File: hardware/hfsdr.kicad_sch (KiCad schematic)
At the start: 8 parts, among them J1 USB_C_Receptacle_USB2.0_16P, U1 SN74CBT3253, U2 XLV320ADC6120IRTER, U3 CH32V30xFxPx, U4 XC6206PxxxMR, Y1 Si5351A-B-GT

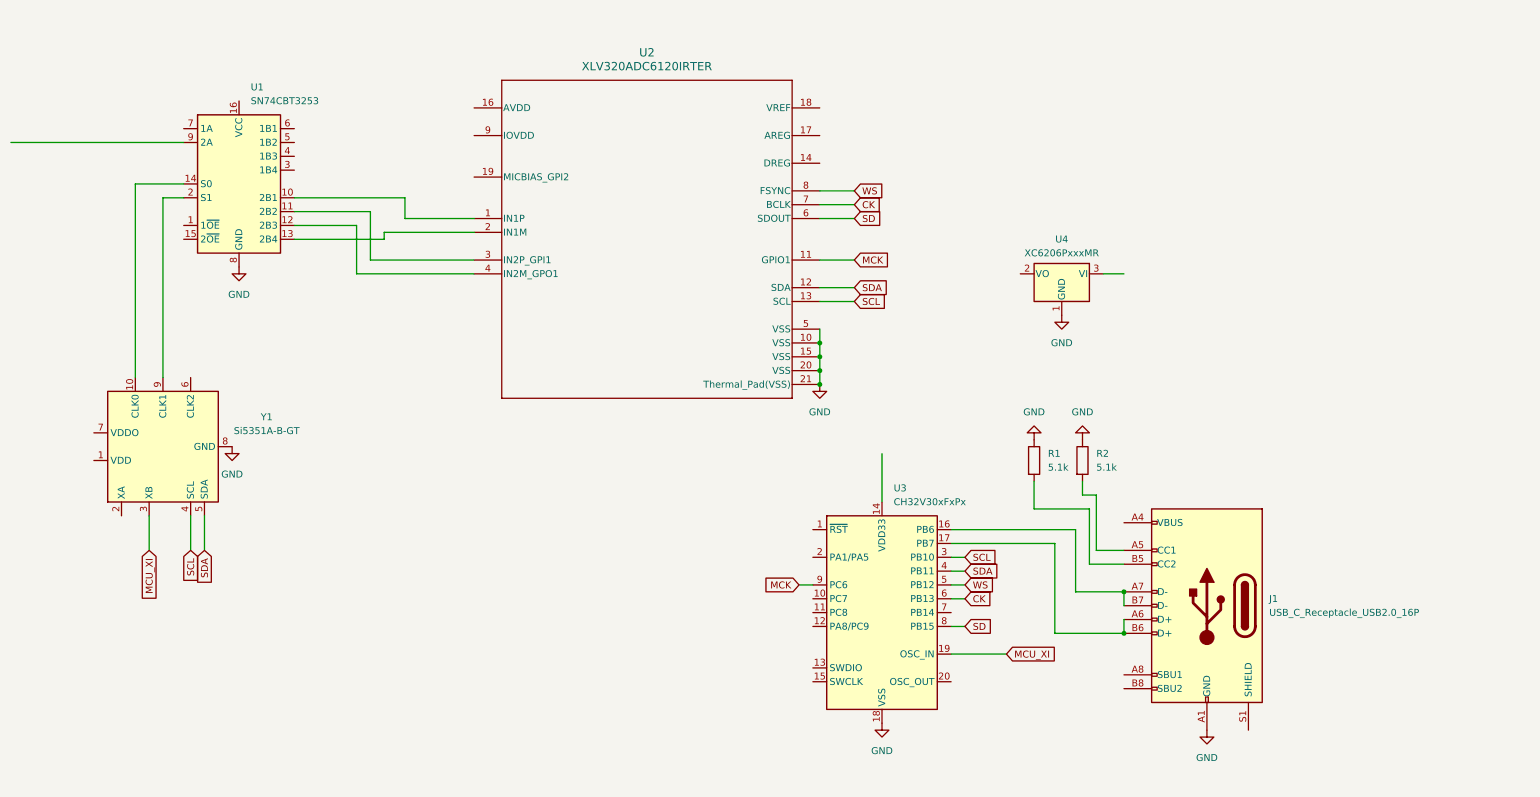
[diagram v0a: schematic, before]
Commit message: Update schematic
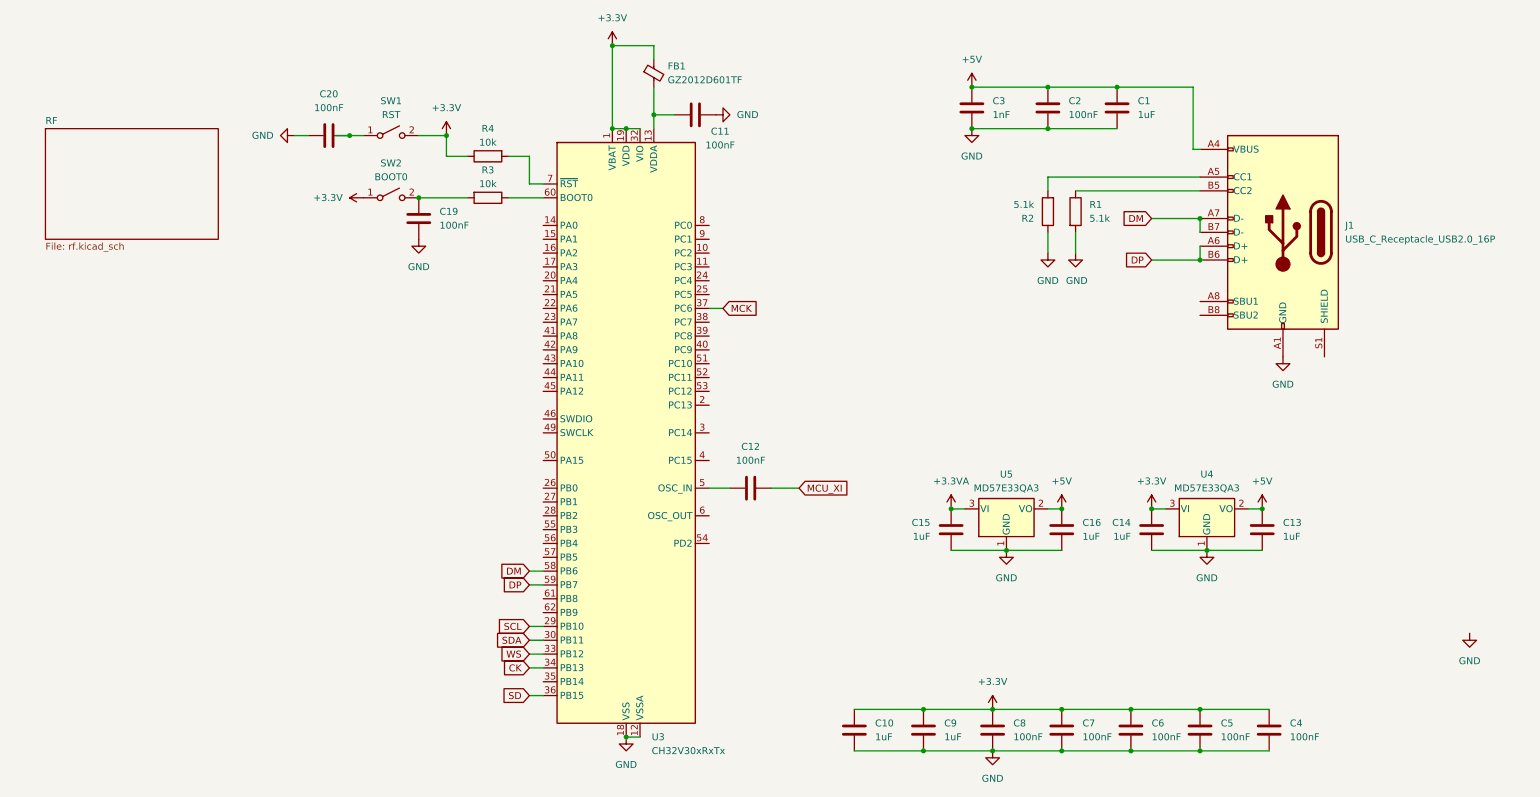
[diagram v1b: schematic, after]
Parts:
- removed U1: SN74CBT3253, Package_SO:TSSOP-16_4.4x5mm_P0.65mm, symbol Analog_Switch:SN74CBT3253
- removed U2: XLV320ADC6120IRTER, RTE0020A-MFG, symbol 2025-06-21_15-05-27:XLV320ADC6120IRTER
- removed U3: CH32V30xFxPx, Package_SO:TSSOP-20_4.4x6.5mm_P0.65mm, symbol MCU_WCH_CH32V3:CH32V30xFxPx
- removed U4: XC6206PxxxMR, Package_TO_SOT_SMD:SOT-23-3, symbol Regulator_Linear:XC6206PxxxMR
- removed Y1: Si5351A-B-GT, Package_SO:MSOP-10_3x3mm_P0.5mm, symbol Oscillator:Si5351A-B-GT
- added C1, C10, C13, C14, C15, C16, C9: 1uF, Capacitor_SMD:C_0805_2012Metric_Pad1.18x1.45mm_HandSolder, symbol Device:C
- added C11, C12, C19, C2, C20, C4, C5, C6, C7, C8: 100nF, Capacitor_SMD:C_0805_2012Metric_Pad1.18x1.45mm_HandSolder, symbol Device:C
- added C3: 1nF, Capacitor_SMD:C_0805_2012Metric_Pad1.18x1.45mm_HandSolder, symbol Device:C
- added FB1: GZ2012D601TF, Inductor_SMD:L_0805_2012Metric_Pad1.05x1.20mm_HandSolder, symbol Device:FerriteBead_Small
- added R3, R4: 10k, Resistor_SMD:R_0603_1608Metric_Pad0.98x0.95mm_HandSolder, symbol Device:R
- added SW1: RST, Button_Switch_SMD:SW_Push_1P1T_XKB_TS-1187A, symbol Switch:SW_SPST
- added SW2: BOOT0, Button_Switch_SMD:SW_Push_1P1T_XKB_TS-1187A, symbol Switch:SW_SPST
- added U3: CH32V30xRxTx, Package_QFP:LQFP-64_10x10mm_P0.5mm, symbol MCU_WCH_CH32V3:CH32V30xRxTx
- added U4, U5: MD57E33QA3, Package_TO_SOT_SMD:SOT-23, symbol Regulator_Linear:TPS7A0520PDBZ
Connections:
- net CK: now also U3.34 (PB13)
- net GND: now also R1.2, C1.2, C10.2, C11.2, C13.2, C14.2, C15.2, C16.2, C19.2, C2.2, C20.1, C3.2, C4.2, C5.2, C6.2, C7.2, C8.2, C9.2, U3.12 (VSSA), U3.18 (VSS), U3.31 (VSS), U3.47 (VSS), U3.63 (VSS), U4.1 (GND), U5.1 (GND); no longer R1.1
- net MCK: now also U3.37 (PC6)
- net MCU_XI: now also C12.2
- net SCL: now also U3.29 (PB10)
- net SD: now also U3.36 (PB15)
- net SDA: now also U3.30 (PB11)
- net WS: now also U3.33 (PB12)
- net at J1.B5 (CC2): now also R1.1; no longer R1.2
- net +5V: now reaches J1.A4 (VBUS), J1.A9 (VBUS), J1.B4 (VBUS), J1.B9 (VBUS)
- net +5V: now also C1.1, C13.1, C16.1, C2.1, C3.1, U4.2 (VO), U5.2 (VO)
- net DP: now reaches J1.A6 (D+), J1.B6 (D+)
- net DP: now also U3.59 (PB7)
- net DM: now reaches J1.A7 (D-), J1.B7 (D-)
- net DM: now also U3.58 (PB6)
- new net: R4.2, U3.7 (~{RST})
- new net: C12.1, U3.5 (OSC_IN)
- new net: C19.1, R3.2, SW2.2 (B)
- new net: C11.1, FB1.2, U3.13 (VDDA)
- new net: R3.1, U3.60 (BOOT0)
- new net: C20.2, SW1.1 (A)
- new net +3.3V: C10.1, C14.1, C4.1, C5.1, C6.1, C7.1, C8.1, C9.1, FB1.1, R4.1, SW1.2 (B), SW2.1 (A), U3.1 (VBAT), U3.19 (VDD), U3.32 (VIO), U3.48 (VDD), U3.64 (VIO), U4.3 (VI)
- new net +3.3VA: C15.1, U5.3 (VI)
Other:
- added sheet RF (rf.kicad_sch)
- moved on the sheet: J1, R1, R2
